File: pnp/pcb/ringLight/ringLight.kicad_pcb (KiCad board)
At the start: 2 copper layers, 39.8 x 48.9 mm, 15 parts, among them J1 Conn_01x03_Male

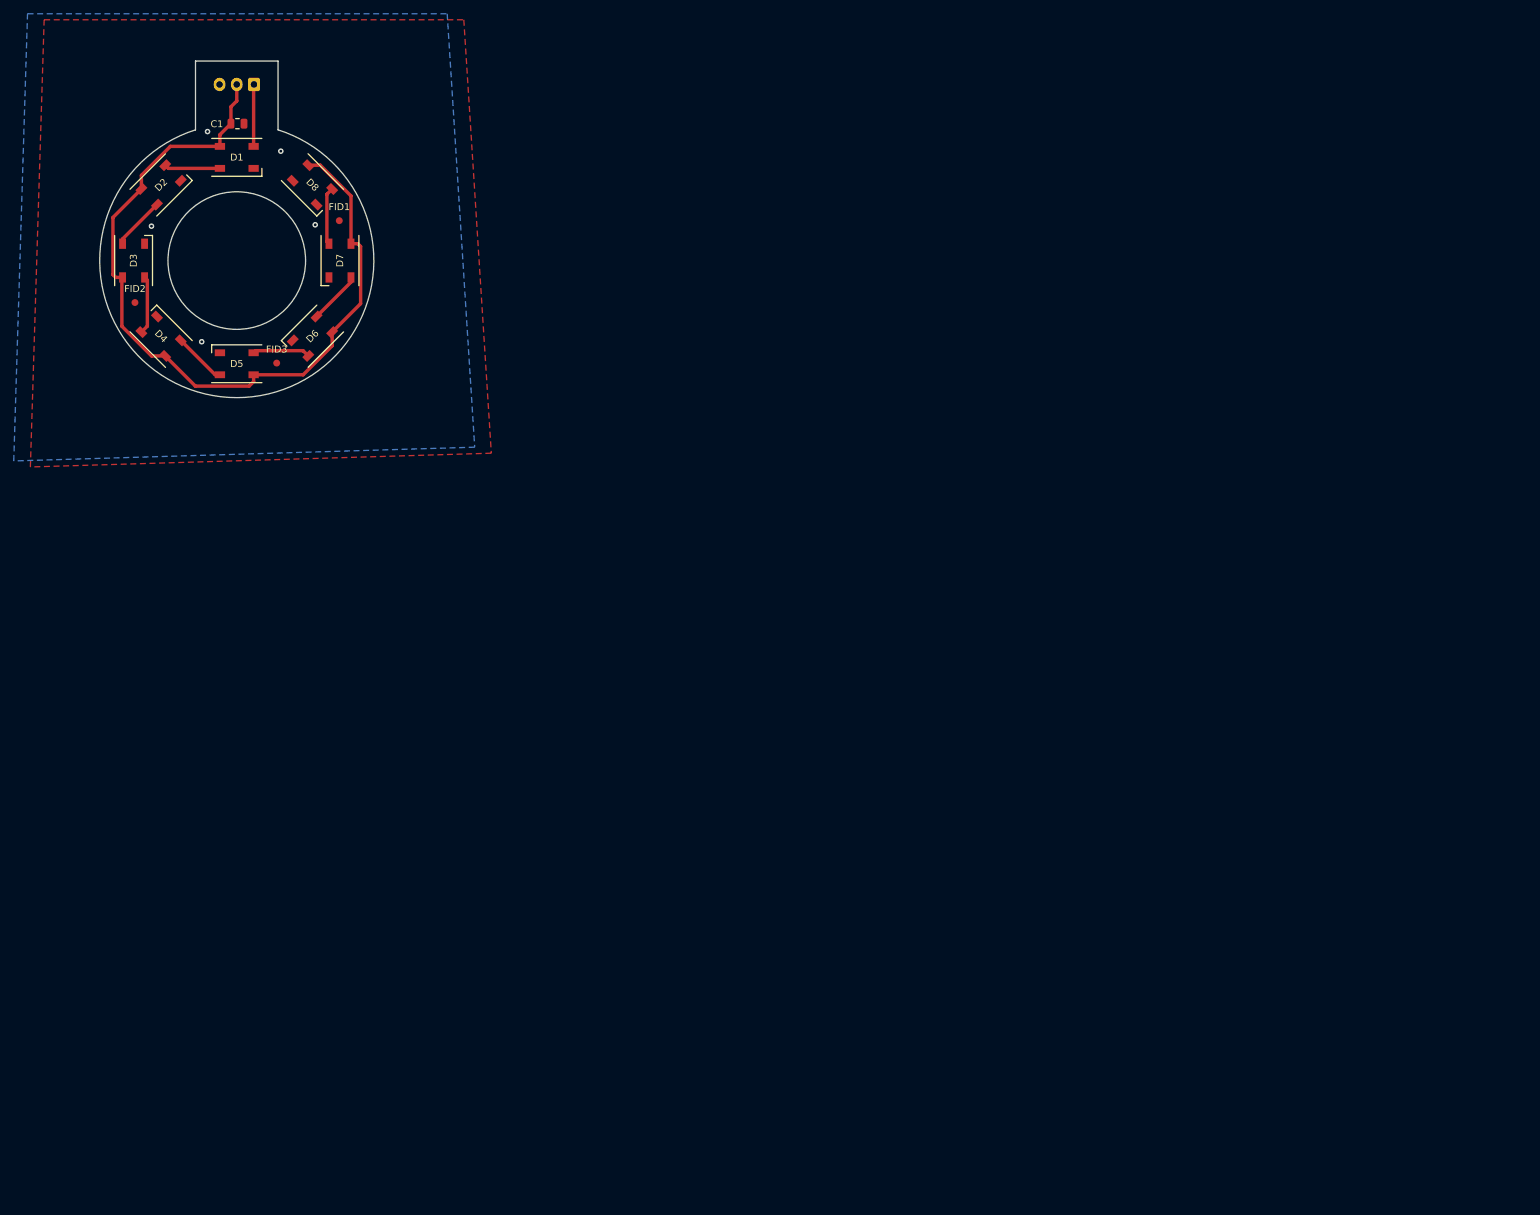
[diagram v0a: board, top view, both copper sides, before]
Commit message: Fix #377
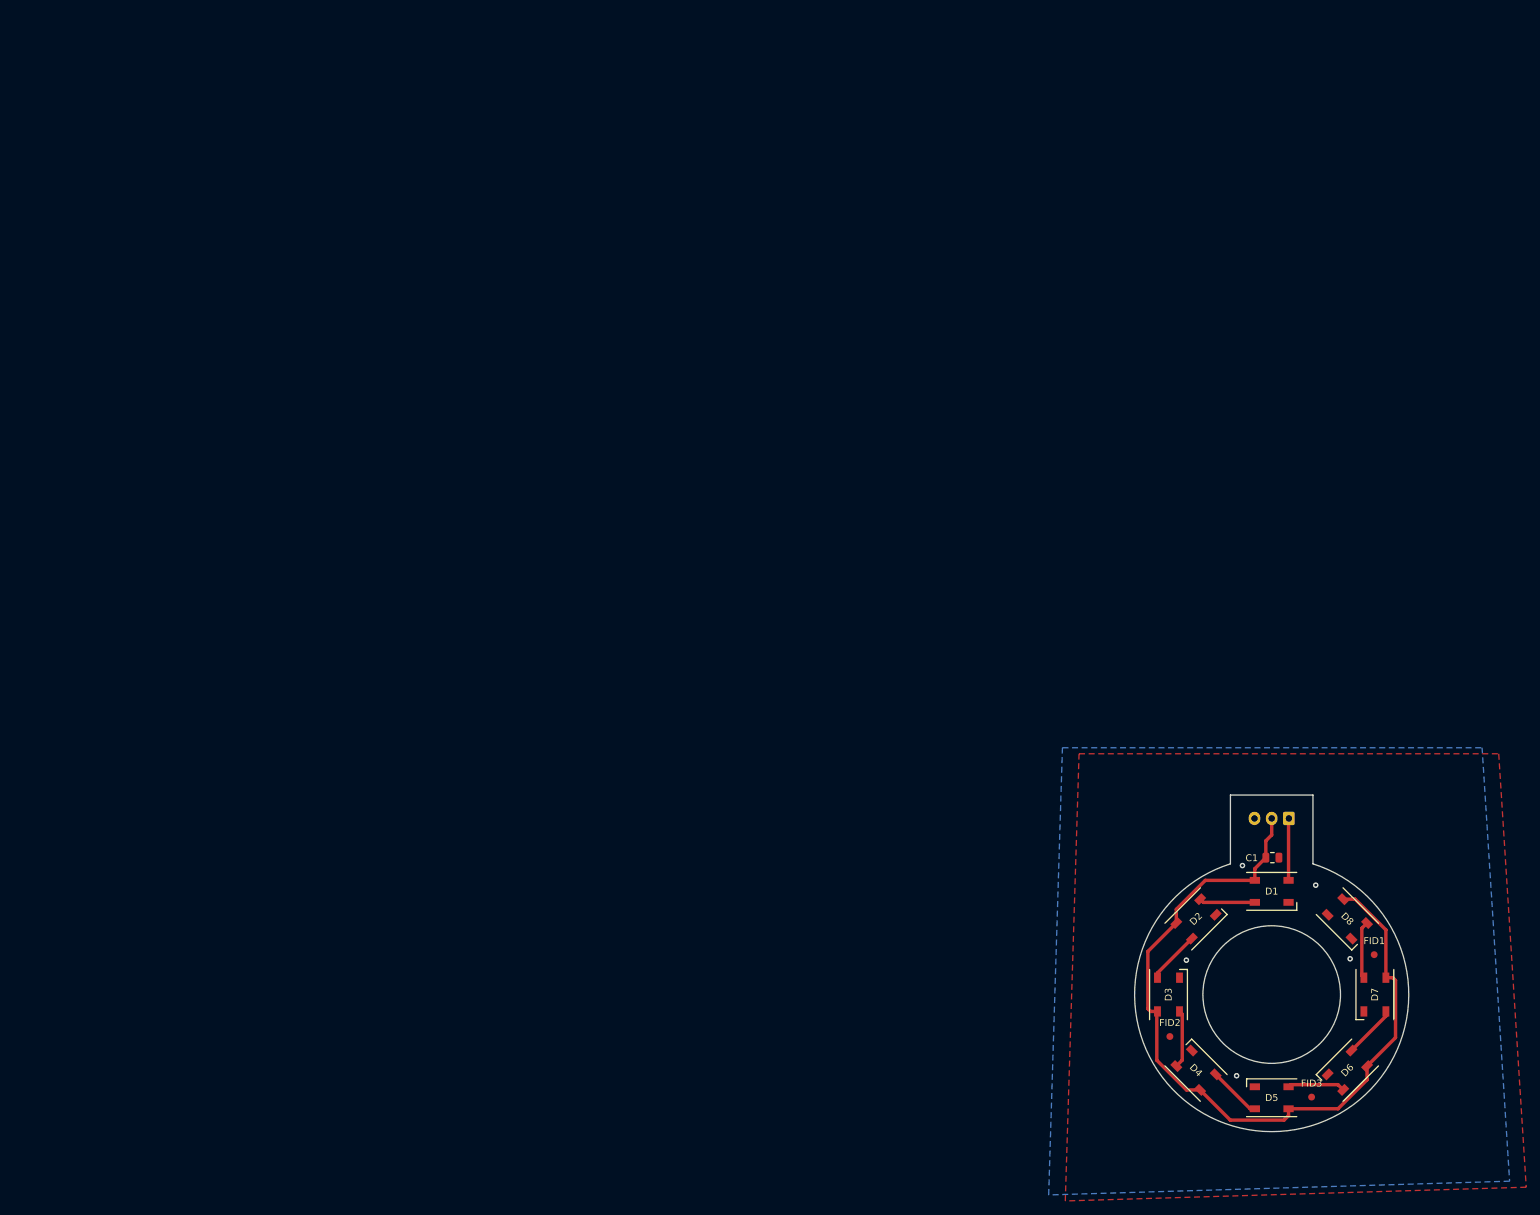
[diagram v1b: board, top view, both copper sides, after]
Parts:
- moved FID2 184.4 mm to (135.6, 112.8)
- moved C1 184.4 mm to (150.5, 86.8)
- moved D1 184.4 mm to (150.4, 91.7)
- moved D2 184.4 mm to (139.4, 95.7)
- moved D3 184.4 mm to (135.4, 106.7)
- moved D4 184.4 mm to (139.4, 117.7)
- moved D5 184.4 mm to (150.4, 121.7)
- moved D6 184.4 mm to (161.4, 117.7)
- moved D7 184.4 mm to (165.4, 106.7)
- moved D8 184.4 mm to (161.4, 95.7)
- moved FID1 184.4 mm to (165.3, 100.9)
- moved FID3 184.4 mm to (156.2, 121.6)
- moved G*** 184.4 mm to (150.6, 89.8)
- moved J1 184.4 mm to (152.9, 81.1)
- moved svg2mod 184.4 mm to (150.5, 94.5)
